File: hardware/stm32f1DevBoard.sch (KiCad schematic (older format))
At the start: 33 parts, among them J1 USB_2, M1 Mounting Hole, M2 Mounting Hole, M3 Mounting Hole, M4 Mounting Hole, P1 JTAG, P2 P20, P3 P20, U1 STM32F102C6, X1 32,768Hz, X2 20MHz

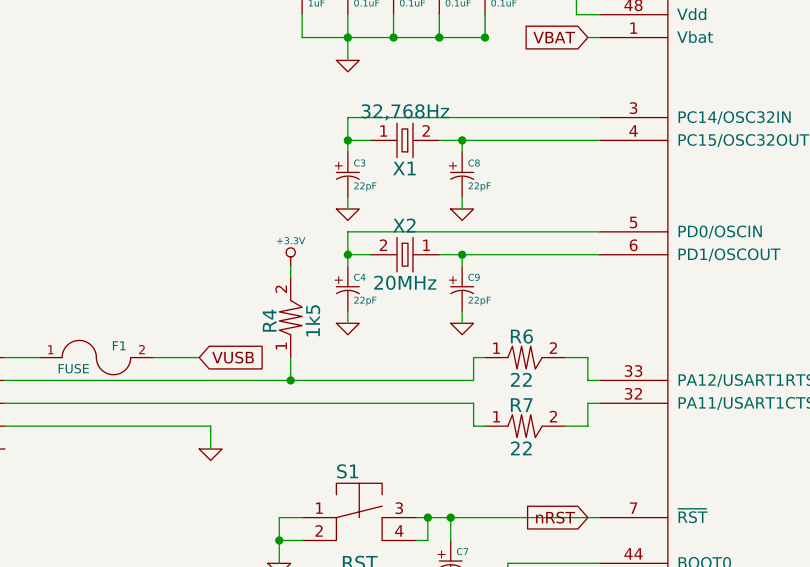
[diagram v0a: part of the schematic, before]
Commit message: updates to schematic
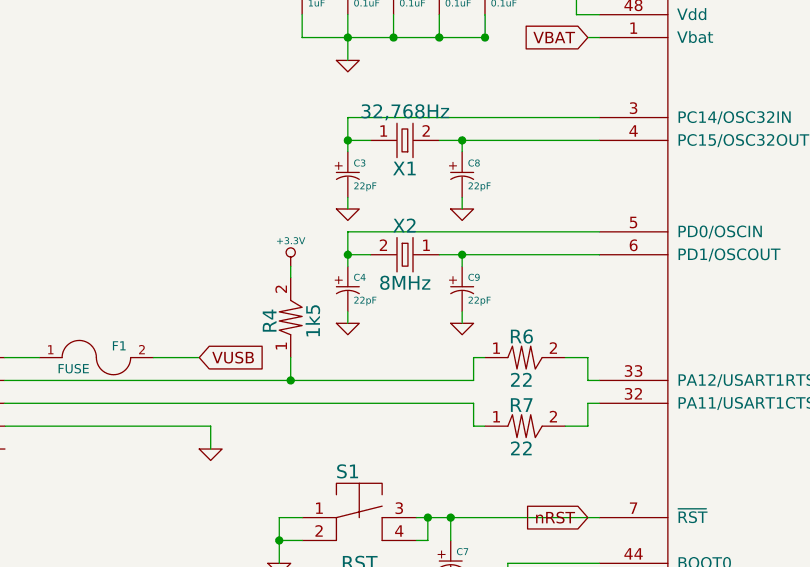
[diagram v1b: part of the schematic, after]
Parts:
- X2: value 20MHz -> 8MHz
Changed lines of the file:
@@
-EESchema Schematic File Version 2  date Thu 17 Jan 2013 09:41:47 PM EST
+EESchema Schematic File Version 2  date Mon 21 Jan 2013 10:28:50 PM EST
 LIBS:userFavorites
 LIBS:power
+LIBS:stm32f1DevBoard-cache
 EELAYER 27 0
 EELAYER END
@@
 Sheet 1 4
 Title ""
-Date "18 jan 2013"
+Date "22 jan 2013"
 Rev ""
 Comp ""
@@
 P 3550 2900
 F 0 "X2" H 3550 3025 60  0000 C CNN
-F 1 "20MHz" H 3550 2775 60  0000 C CNN
+F 1 "8MHz" H 3550 2775 60  0000 C CNN
 	1    3550 2900
 	1    0    0    -1
